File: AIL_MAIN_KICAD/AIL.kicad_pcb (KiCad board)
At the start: 2 copper layers, 71.9 x 33.4 mm, 25 parts, among them IC1 LT8315, J1 Conn_01x02_Female, J2 Conn_01x02_Female

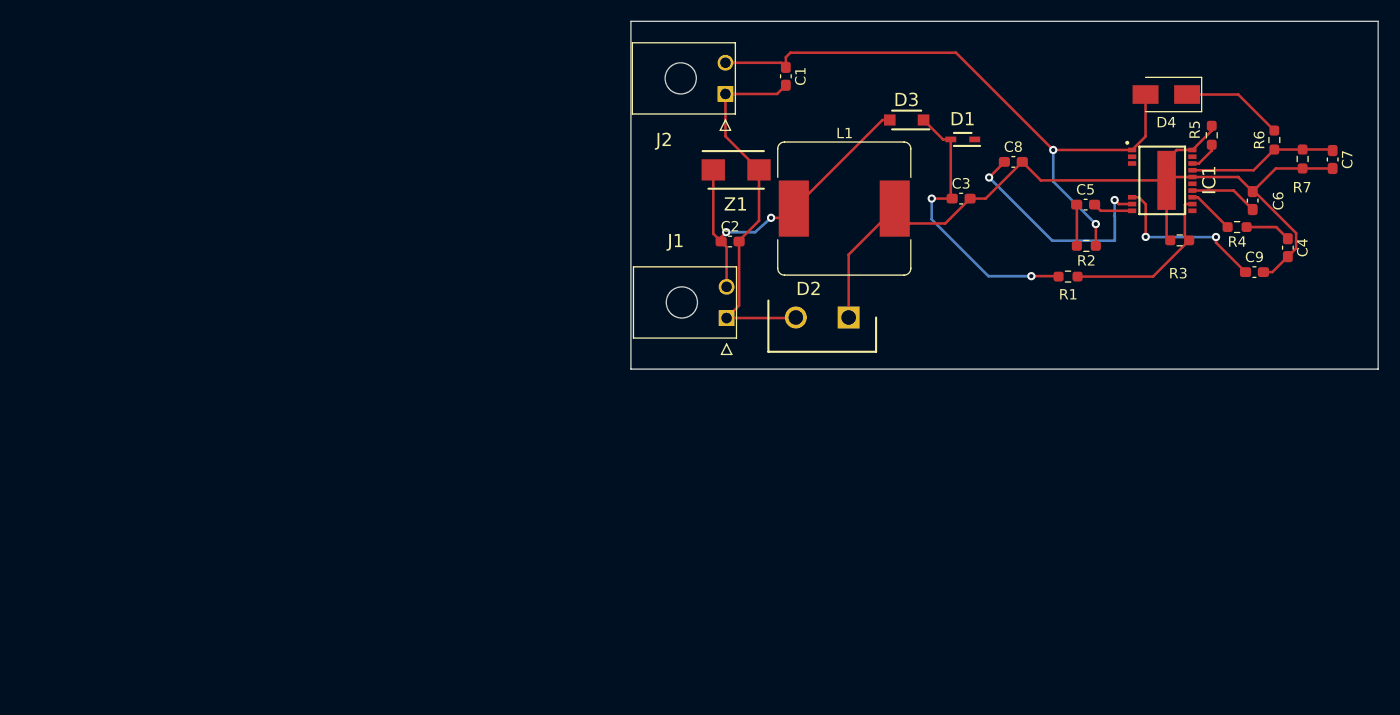
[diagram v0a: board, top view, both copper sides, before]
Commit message: Updating main board
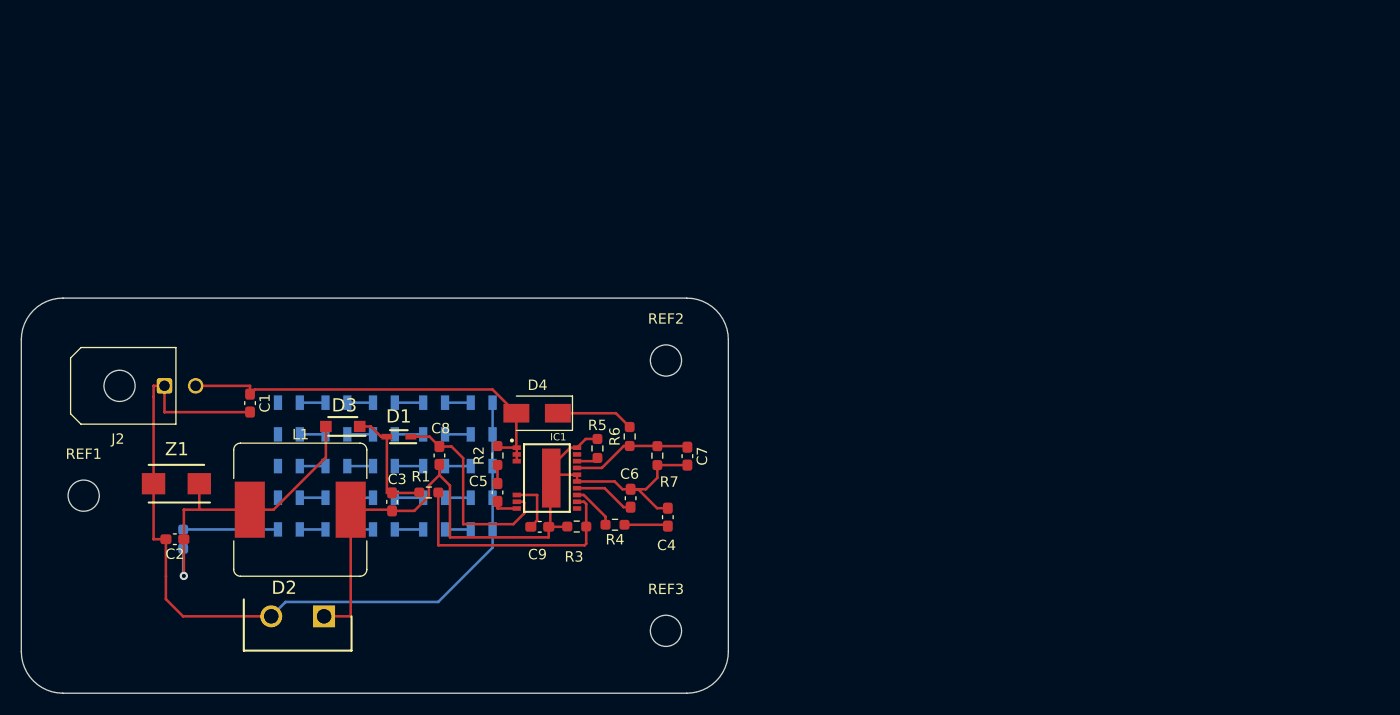
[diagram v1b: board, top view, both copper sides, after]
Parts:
- removed J1: Conn_01x02_Female, 2155760-1002:215760-YY02
- added D10: LED, AIL_MAIN_FOOT:LEDC2012X100N, B.Cu at (141.7, 92.2)
- added D11: LED, AIL_MAIN_FOOT:LEDC2012X100N, B.Cu at (146.3, 92.2)
- added D12: LED, AIL_MAIN_FOOT:LEDC2012X100N, B.Cu at (150.9, 92.2)
- added D13: LED, AIL_MAIN_FOOT:LEDC2012X100N, B.Cu at (155.7, 92.2)
- added D14: LED, AIL_MAIN_FOOT:LEDC2012X100N, B.Cu at (160.3, 92.2)
- added D15: LED, AIL_MAIN_FOOT:LEDC2012X100N, B.Cu at (141.7, 89.2)
- added D16: LED, AIL_MAIN_FOOT:LEDC2012X100N, B.Cu at (146.3, 89.2)
- added D17: LED, AIL_MAIN_FOOT:LEDC2012X100N, B.Cu at (150.9, 89.2)
- added D18: LED, AIL_MAIN_FOOT:LEDC2012X100N, B.Cu at (155.7, 89.2)
- added D19: LED, AIL_MAIN_FOOT:LEDC2012X100N, B.Cu at (160.3, 89.2)
- added D20: LED, AIL_MAIN_FOOT:LEDC2012X100N, B.Cu at (141.7, 86.1)
- added D21: LED, AIL_MAIN_FOOT:LEDC2012X100N, B.Cu at (146.3, 86.1)
- added D22: LED, AIL_MAIN_FOOT:LEDC2012X100N, B.Cu at (150.9, 86.1)
- added D23: LED, AIL_MAIN_FOOT:LEDC2012X100N, B.Cu at (155.7, 86.1)
- added D24: LED, AIL_MAIN_FOOT:LEDC2012X100N, B.Cu at (160.3, 86.1)
- added D25: LED, AIL_MAIN_FOOT:LEDC2012X100N, B.Cu at (141.7, 83.1)
- added D26: LED, AIL_MAIN_FOOT:LEDC2012X100N, B.Cu at (146.3, 83.1)
- added D27: LED, AIL_MAIN_FOOT:LEDC2012X100N, B.Cu at (150.9, 83.1)
- added D28: LED, AIL_MAIN_FOOT:LEDC2012X100N, B.Cu at (155.7, 83.1)
- added D29: LED, AIL_MAIN_FOOT:LEDC2012X100N, B.Cu at (160.3, 83.1)
- added D5: LED, AIL_MAIN_FOOT:LEDC2012X100N, B.Cu at (141.7, 95.2)
- added D6: LED, AIL_MAIN_FOOT:LEDC2012X100N, B.Cu at (146.3, 95.2)
- added D7: LED, AIL_MAIN_FOOT:LEDC2012X100N, B.Cu at (150.9, 95.2)
- added D8: LED, AIL_MAIN_FOOT:LEDC2012X100N, B.Cu at (155.7, 95.2)
- added D9: LED, AIL_MAIN_FOOT:LEDC2012X100N, B.Cu at (160.3, 95.2)
- added R8: 20, Resistor_SMD:R_0603_1608Metric_Pad0.98x0.95mm_HandSolder, B.Cu at (131.6, 96.2)
- added REF1: MountingHole_3mm, MountingHole:MountingHole_3mm, F.Cu at (122.0, 92.0)
- added REF2: MountingHole_3mm, MountingHole:MountingHole_3mm, F.Cu at (178.0, 79.0)
- added REF3: MountingHole_3mm, MountingHole:MountingHole_3mm, F.Cu at (178.0, 105.0)
- J2: footprint 2155760-1002:215760-YY02 -> Connector_Molex:Molex_Micro-Fit_3.0_43045-0200_2x01_P3.00mm_Horizontal
- moved C9 73.0 mm to (165.9, 95.0)
- moved C7 68.3 mm to (180.1, 88.2)
- moved R7 68.3 mm to (177.2, 88.2)
- moved R6 68.2 mm to (174.5, 86.3)
- moved D4 67.8 mm to (165.6, 84.1)
- moved C6 66.3 mm to (174.6, 92.2)
- moved R4 66.3 mm to (173.1, 94.8)
- moved R5 66.3 mm to (171.4, 87.5)
- moved IC1 65.7 mm to (166.5, 90.3)
- moved C4 65.0 mm to (178.2, 94.1), turned to 90 degrees
- moved R1 64.9 mm to (155.2, 91.7)
- moved R3 64.2 mm to (169.4, 95.0)
- moved C5 63.0 mm to (161.8, 91.7), turned to -90 degrees
- moved C3 62.0 mm to (151.7, 92.6), turned to -90 degrees
- moved C8 62.0 mm to (156.2, 88.1), turned to -90 degrees
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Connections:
- net /12V renamed +12V
- IC1 pad 15: unconnected-(IC1-Pad15) -> ICGND
- IC1 pad 2: unconnected-(IC1-Pad2) -> HV1
- IC1 pad 3: unconnected-(IC1-Pad3) -> HV1
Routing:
- net GND: track 37.0 -> 82.3 mm
- net HV1: track 61.1 -> 39.0 mm, vias 2 -> 0
- net Net-(C3-Pad1): track 27.8 -> 11.6 mm, vias 2 -> 0
- net Net-(C9-Pad1): track 16.0 -> 5.27 mm, vias 2 -> 0
- net Net-(D10-Pad2): track 0.00 -> 9.09 mm
- net ICGND: track 85.1 -> 76.1 mm
- net HV3: track 16.6 -> 24.2 mm
- net +12V: track 33.2 -> 30.1 mm, vias 2 -> 1
- net Net-(C7-Pad1): track 14.4 -> 11.5 mm
- net Net-(D7-Pad1): track 0.00 -> 2.73 mm
- net Net-(D27-Pad1): track 0.00 -> 2.73 mm
- net Net-(D22-Pad1): track 0.00 -> 2.73 mm
- net Net-(D17-Pad1): track 0.00 -> 2.73 mm
- net Net-(D12-Pad1): track 0.00 -> 2.73 mm
- net Net-(D8-Pad1): track 0.00 -> 2.47 mm
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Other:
- board size 71.9 x 33.4 mm -> 68 x 38 mm
